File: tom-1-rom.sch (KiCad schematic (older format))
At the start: 2 parts, among them J10 Conn_02x08_Top_Bottom, U20 27C1024

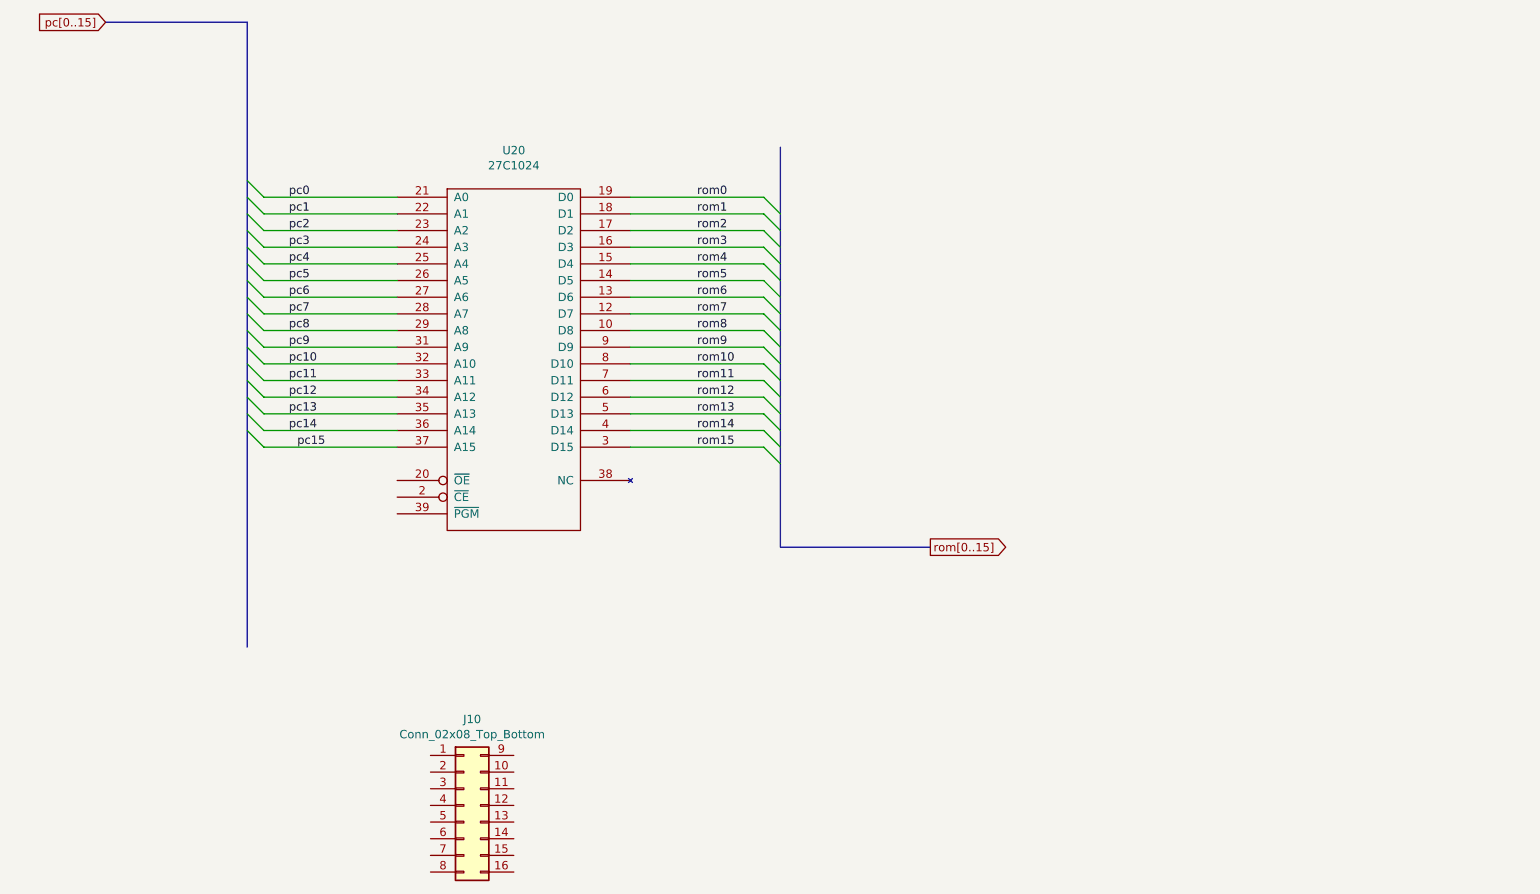
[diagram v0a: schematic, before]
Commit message: Next level
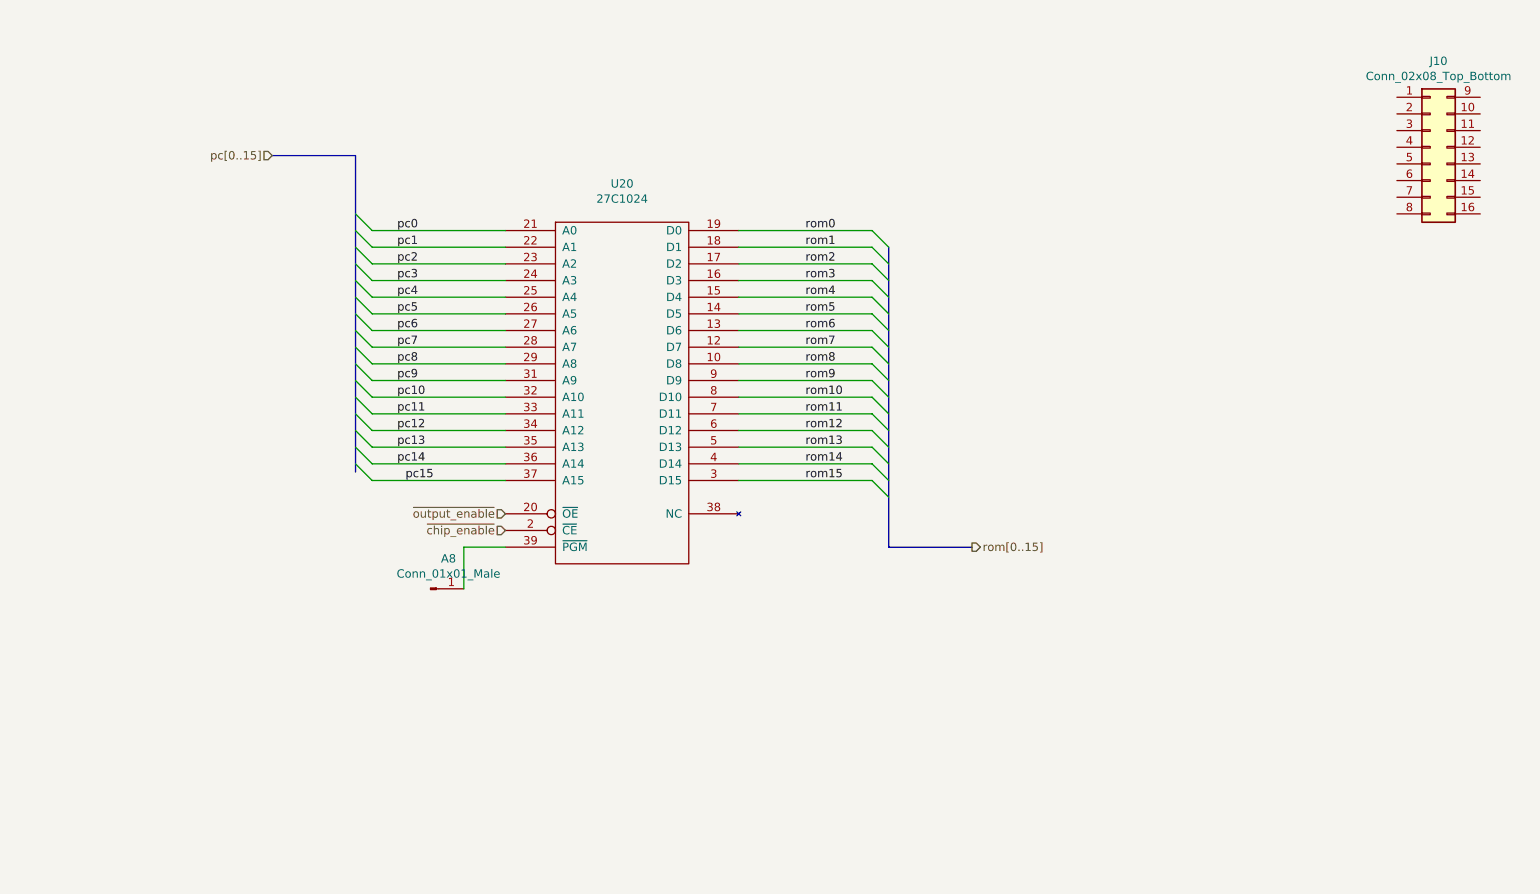
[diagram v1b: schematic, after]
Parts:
- added A8: Conn_01x01_Male, Connector_PinHeader_2.54mm:PinHeader_1x01_P2.54mm_Vertical, symbol Connector:Conn_01x01_Male
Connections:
- net ~chip_enable~: now reaches U20.2 (~CE)
- net ~output_enable~: now reaches U20.20 (~OE)
- net at U20.39 (~PGM): now also A8.1 (Pin_1)
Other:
- moved on the sheet: J10, U20
